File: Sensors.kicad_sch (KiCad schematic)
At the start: 1 part, among them IC1 ICM-42688-P

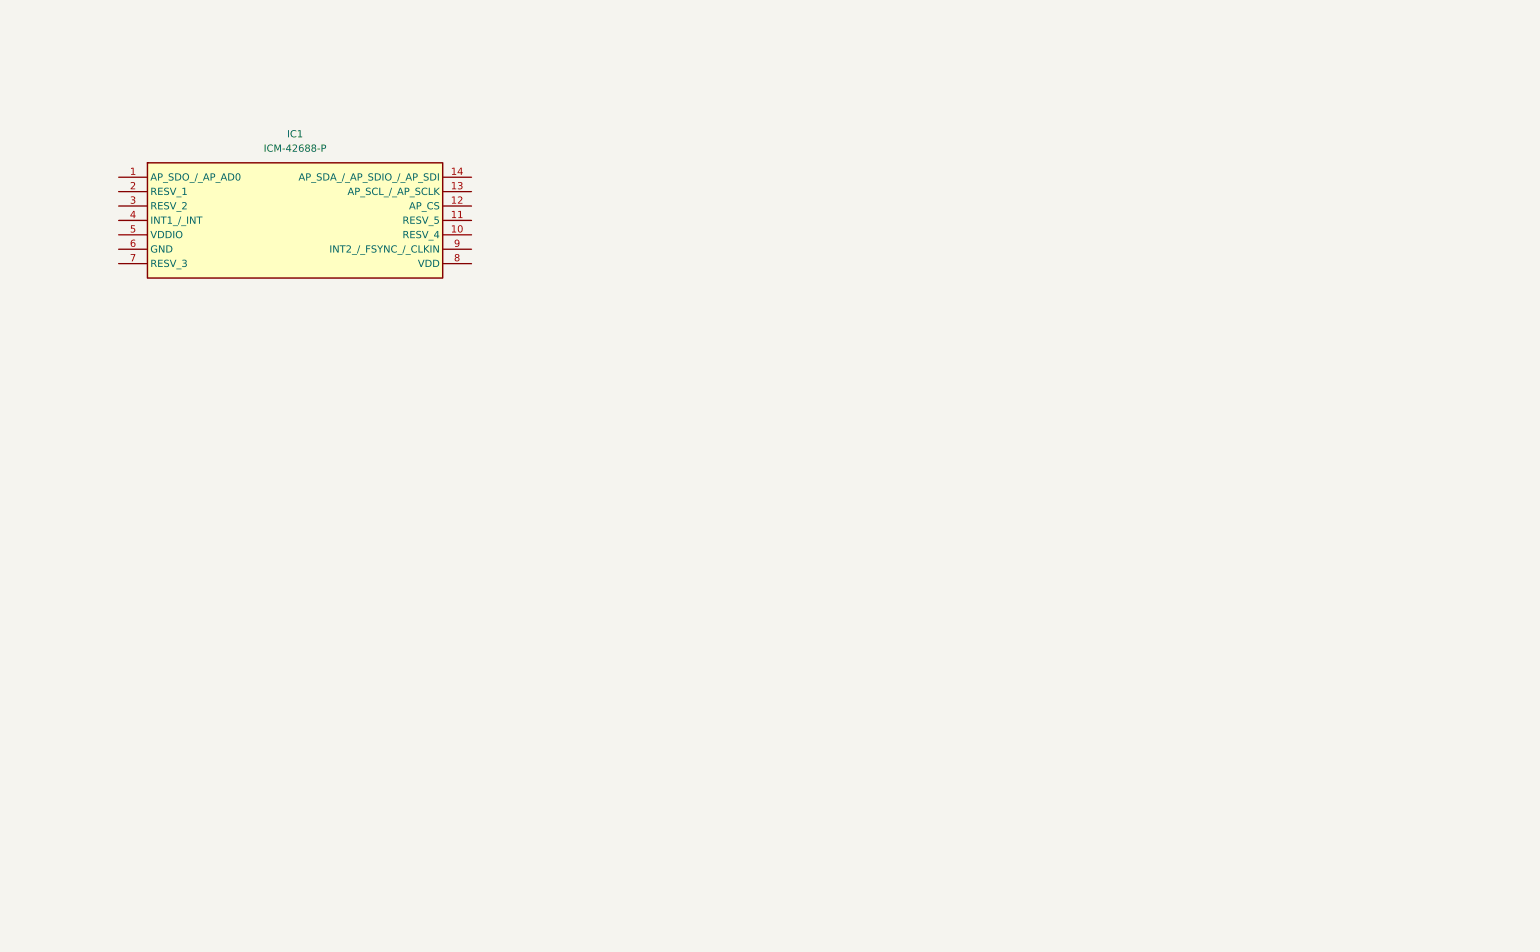
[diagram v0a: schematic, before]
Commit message: Update SCH
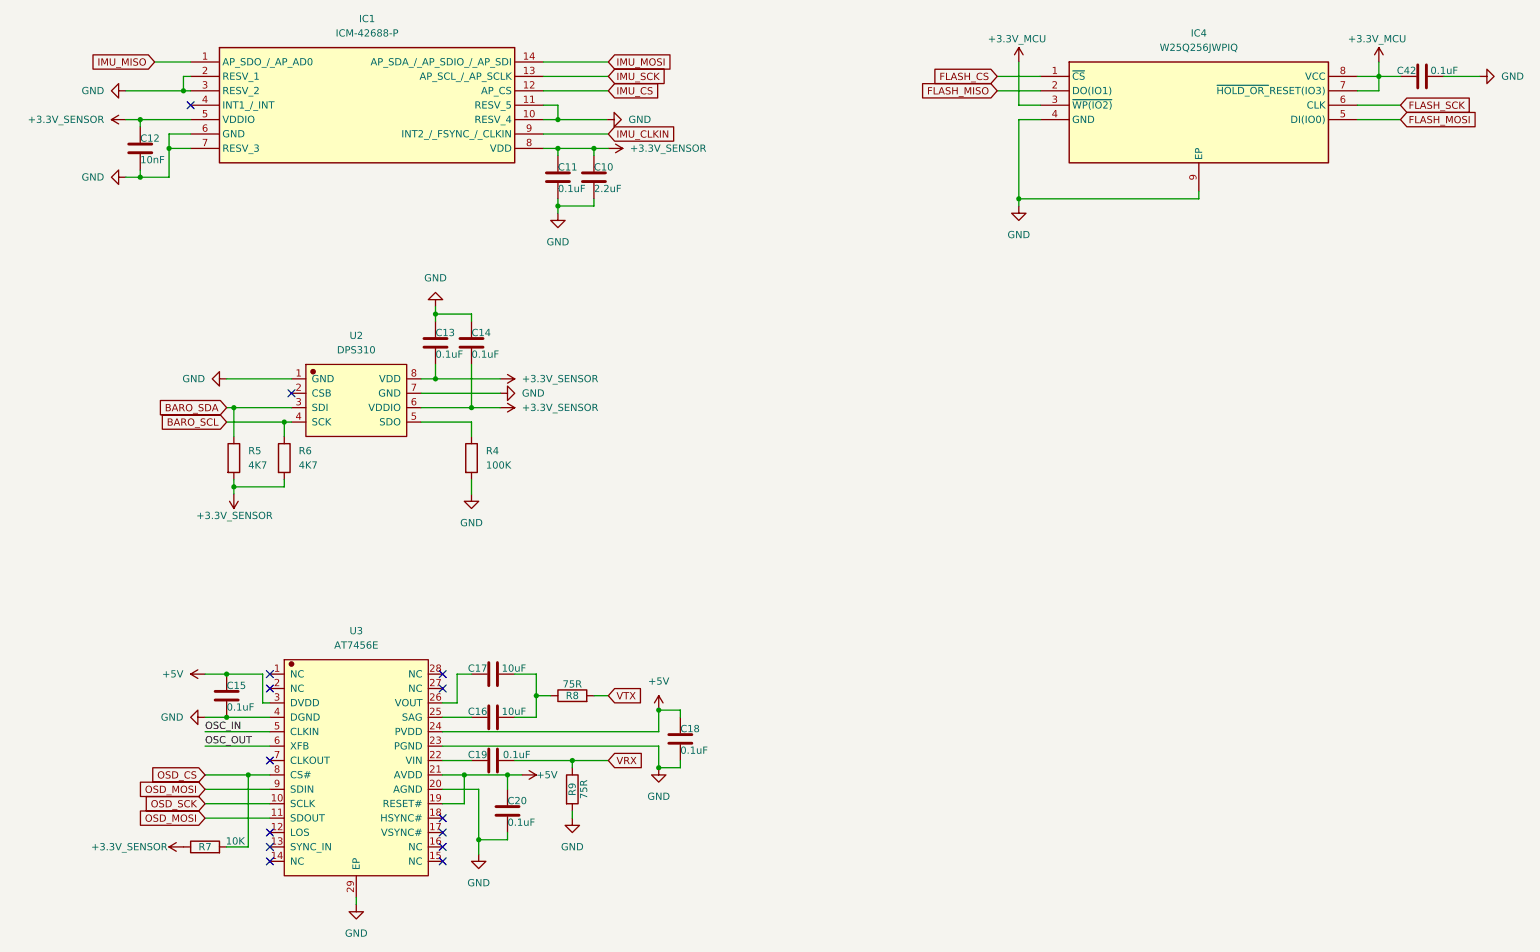
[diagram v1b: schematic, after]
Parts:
- added C10: 2.2uF, symbol Library:C
- added C11, C13, C14, C15, C18, C19, C20, C42: 0.1uF, symbol Library:C
- added C12: 10nF, symbol Library:C
- added C16, C17: 10uF, symbol Library:C
- added IC4: W25Q256JWPIQ, SON127P600X500X80-9N-D, symbol Library:W25Q256JWPIQ
- added R4: 100K, symbol Library:R
- added R5, R6: 4K7, symbol Library:R
- added R7: 10K, symbol Library:R
- added R8, R9: 75R, symbol Library:R
- added U2: DPS310, SamacSys_Parts:WLGA-8_L2.5-W2.0-P0.65-TR_DPS422, symbol Library:DPS310
- added U3: AT7456E, SamacSys_Parts:TSSOP-28_L9.7-W4.4-P0.65-LS6.4-BL-EP-2, symbol Library:AT7456E
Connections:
- net IMU_MISO: now reaches IC1.1 (AP_SDO_/_AP_AD0)
- net GND: now reaches IC1.10 (RESV_4)
- net GND: now also IC1.11 (RESV_5), IC1.2 (RESV_1), IC1.3 (RESV_2), IC1.6 (GND), IC1.7 (RESV_3), C10.2, C11.2, C12.2, C13.1, C14.1, C15.2, C18.2, C20.2, C42.2, IC4.4 (GND), IC4.9 (EP), R4.2, R9.2, U2.1 (GND), U2.7 (GND), U3.20 (AGND), U3.23 (PGND), U3.29 (EP), U3.4 (DGND)
- net IMU_CS: now reaches IC1.12 (AP_CS)
- net IMU_SCK: now reaches IC1.13 (AP_SCL_/_AP_SCLK)
- net IMU_MOSI: now reaches IC1.14 (AP_SDA_/_AP_SDIO_/_AP_SDI)
- net +3.3V_SENSOR: now reaches IC1.5 (VDDIO)
- net +3.3V_SENSOR: now also IC1.8 (VDD), C10.1, C11.1, C12.1, C13.2, C14.2, R5.2, R6.2, R7.1, U2.6 (VDDIO), U2.8 (VDD)
- net IMU_CLKIN: now reaches IC1.9 (INT2_/_FSYNC_/_CLKIN)
- new net: C16.2, C17.2, R8.1
- new net: R4.1, U2.5 (SDO)
- new net: C17.1, U3.26 (VOUT)
- new net: C19.1, U3.22 (VIN)
- new net: C16.1, U3.25 (SAG)
- new net +3.3V_MCU: C42.1, IC4.3 (~{WP(IO2)}), IC4.7 (~{HOLD_OR_}RESET(IO3)), IC4.8 (VCC)
- new net +5V: C15.1, C18.1, C20.1, U3.19 (RESET#), U3.21 (AVDD), U3.24 (PVDD), U3.3 (DVDD)
- new net BARO_SCL: R6.1, U2.4 (SCK)
- new net BARO_SDA: R5.1, U2.3 (SDI)
- new net FLASH_CS: IC4.1 (~{CS})
- new net FLASH_MISO: IC4.2 (DO(IO1))
- new net FLASH_MOSI: IC4.5 (DI(IO0))
- new net FLASH_SCK: IC4.6 (CLK)
- new net OSC_IN: U3.5 (CLKIN)
- new net OSC_OUT: U3.6 (XFB)
- new net OSD_CS: R7.2, U3.8 (CS#)
- new net OSD_MOSI: U3.11 (SDOUT), U3.9 (SDIN)
- new net OSD_SCK: U3.10 (SCLK)
- new net VRX: C19.2, R9.1
- new net VTX: R8.2
- no-connect marks 0 -> 14
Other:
- moved on the sheet: IC1
